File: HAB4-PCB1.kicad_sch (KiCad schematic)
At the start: 16 parts, among them J1 Barrel_Jack_Switch

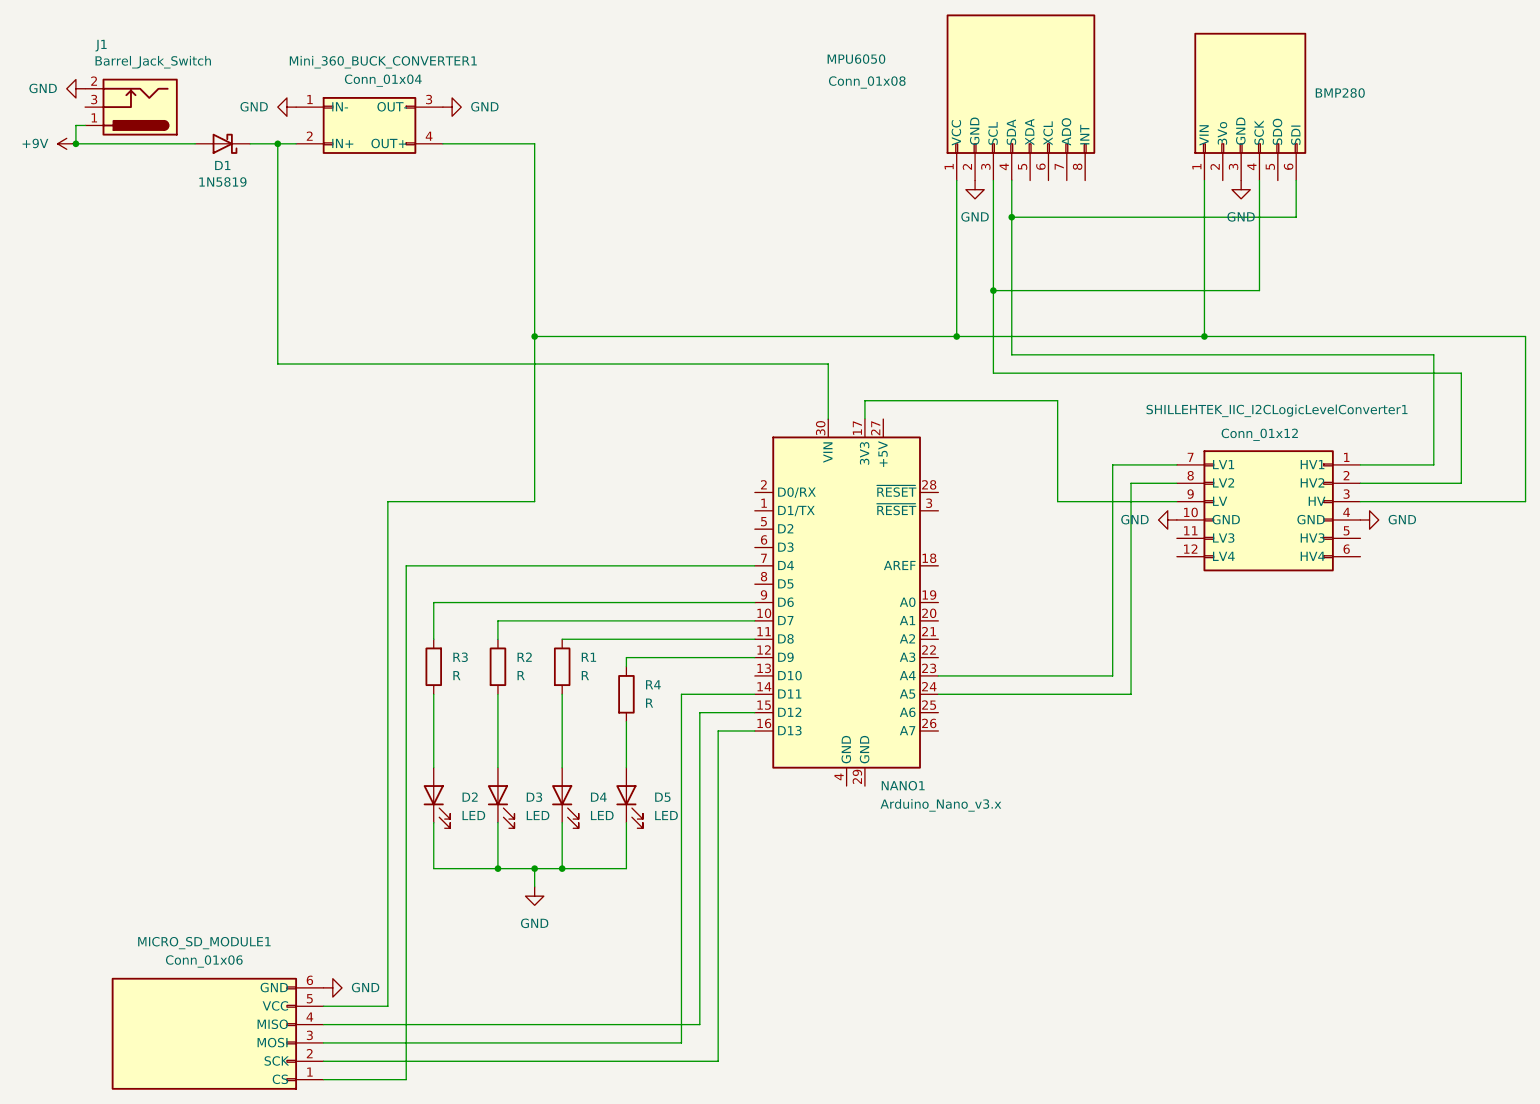
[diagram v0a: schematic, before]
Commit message: Jumper cables and other
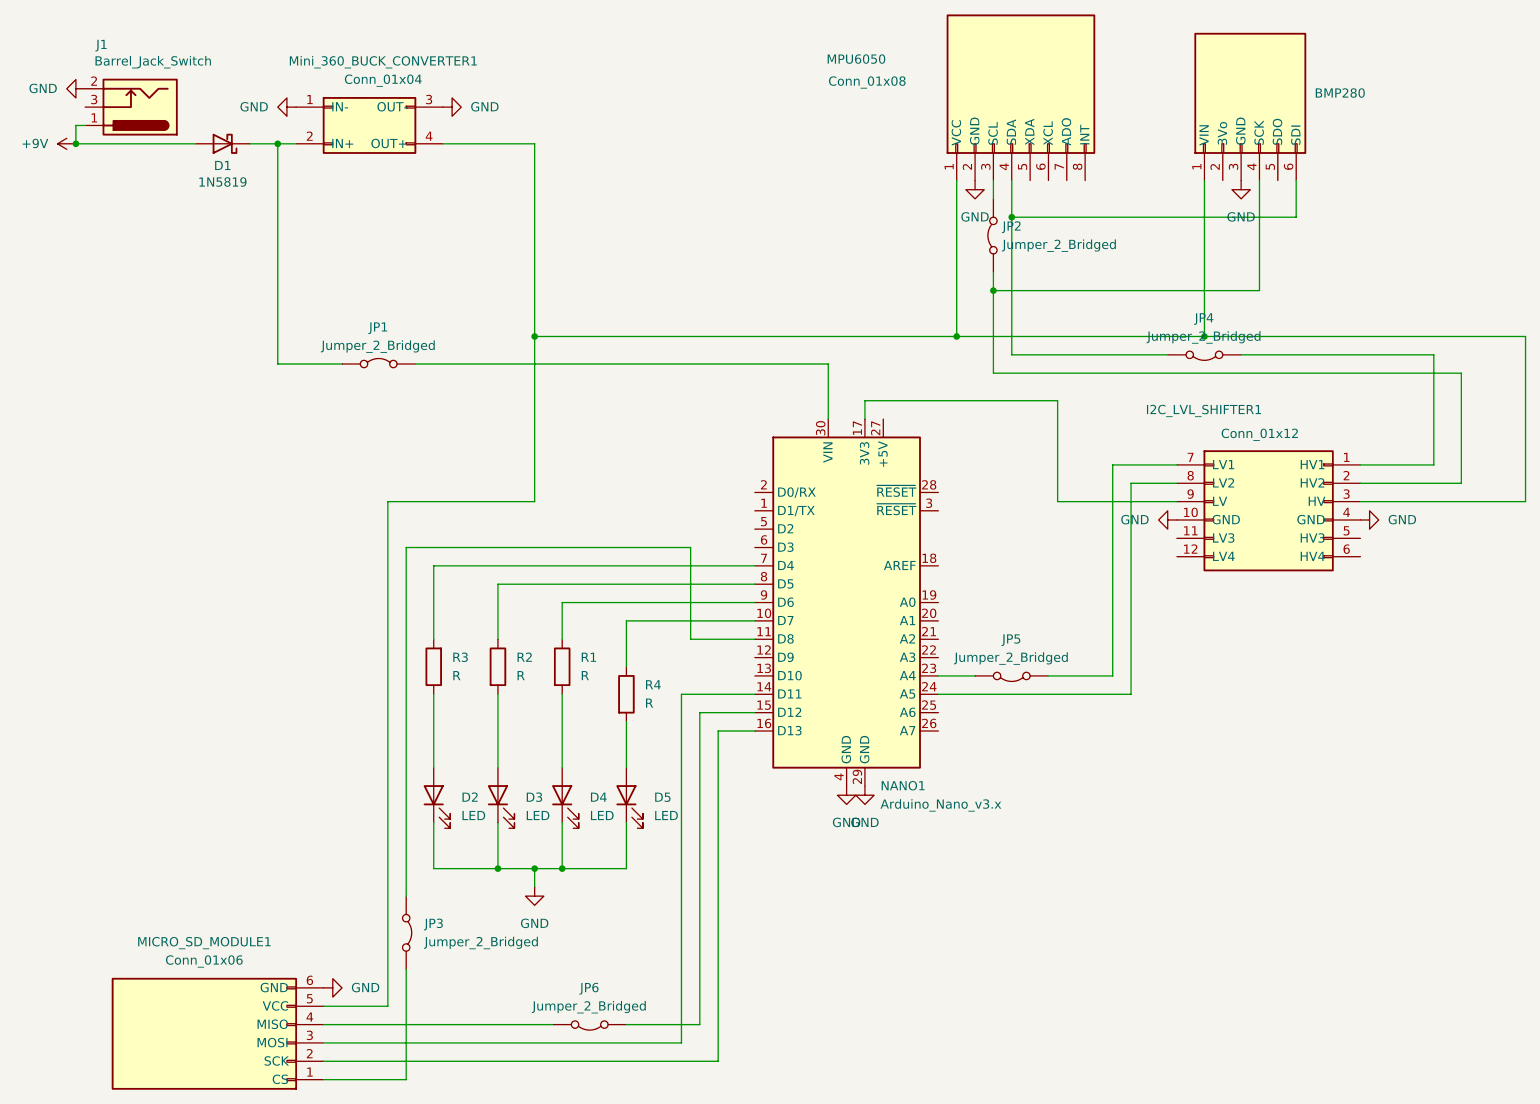
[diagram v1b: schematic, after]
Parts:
- added JP1, JP2, JP4, JP5: Jumper_2_Bridged, My_Footprints2:6mm_jumper, symbol Jumper:Jumper_2_Bridged
- added JP3, JP6: Jumper_2_Bridged, My_Footprints2:8mm_jumper, symbol Jumper:Jumper_2_Bridged
- renumbered SHILLEHTEK_IIC_I2CLogicLevelConverter1 to I2C_LVL_SHIFTER1
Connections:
- net GND: now also NANO1.29 (GND), NANO1.4 (GND)
- net at R1.1: now also NANO1.9 (D6); no longer NANO1.11 (D8)
- net at BMP280.6 (SDI), MPU6050.4 (SDA): now also JP4.2 (B); no longer I2C_LVL_SHIFTER1.1 (HV1)
- net at BMP280.4 (SCK), I2C_LVL_SHIFTER1.2 (HV2): now also JP2.1 (A); no longer MPU6050.3 (SCL)
- net at I2C_LVL_SHIFTER1.7 (LV1): now also JP5.1 (A); no longer NANO1.23 (A4)
- net at D1.1 (K), Mini_360_BUCK_CONVERTER1.2 (IN+): now also JP1.1 (A); no longer NANO1.30 (VIN)
- net at R2.1: now also NANO1.8 (D5); no longer NANO1.10 (D7)
- net at R4.1: now also NANO1.10 (D7); no longer NANO1.12 (D9)
- net at MICRO_SD_MODULE1.1 (CS): now also JP3.2 (B); no longer NANO1.7 (D4)
- net at NANO1.15 (D12): now also JP6.1 (A); no longer MICRO_SD_MODULE1.4 (MISO)
- net at R3.2: now also NANO1.7 (D4); no longer NANO1.9 (D6)
- new net: JP5.2 (B), NANO1.23 (A4)
- new net: I2C_LVL_SHIFTER1.1 (HV1), JP4.1 (A)
- new net: JP2.2 (B), MPU6050.3 (SCL)
- new net: JP6.2 (B), MICRO_SD_MODULE1.4 (MISO)
- new net: JP3.1 (A), NANO1.11 (D8)
- new net: JP1.2 (B), NANO1.30 (VIN)
